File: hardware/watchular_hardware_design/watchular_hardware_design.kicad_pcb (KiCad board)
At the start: 4 copper layers, 55.5 x 22.9 mm, 90 parts, among them J1 USB4105-GF-A, J2 665102131822, J3 TSW-116-07-H-S, J4 TSW-116-07-H-S, Q1 BSS123, Q2 BSS123, Q3 BSS123, Q4 BSS123, T1 DMG1013UW-7, U1 MCP73832T-2DCI/OT, U2 ESP32-C3FH4, U3 MIC5524-3.3YMT-TZ, U4 W25Q16JVSSIQ, U5 TL3305AF260QG, U6 TL3305AF260QG, Y1 40MHz

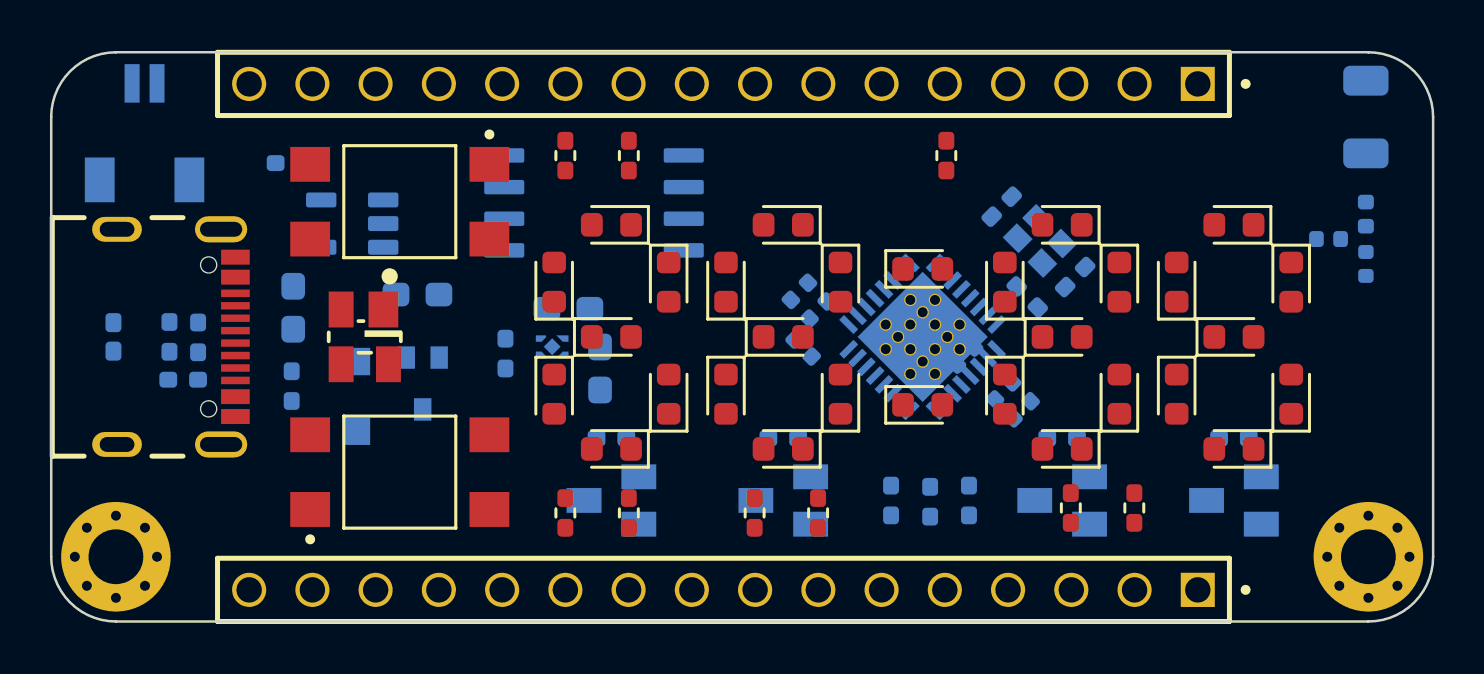
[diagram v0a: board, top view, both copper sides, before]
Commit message: Let the routing begin.
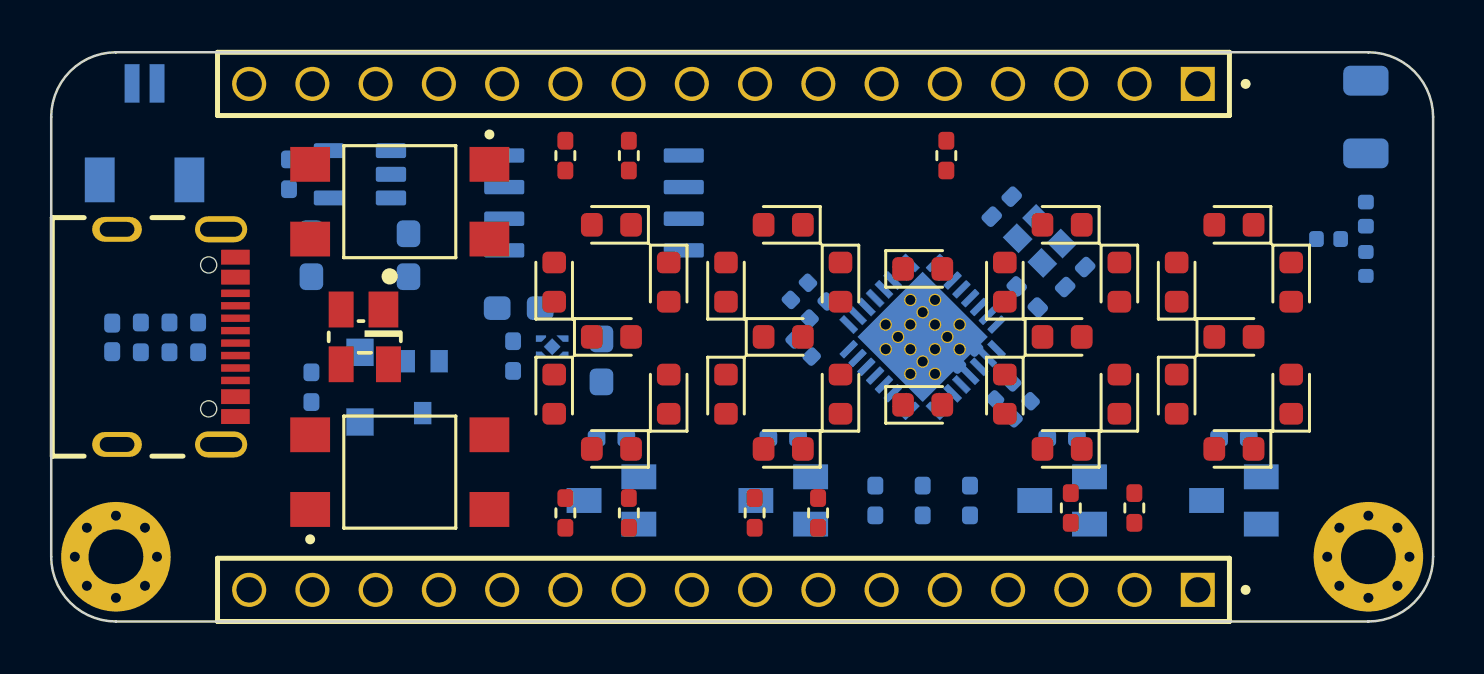
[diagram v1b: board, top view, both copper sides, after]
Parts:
- moved R5 2.40 mm to (93.6, 121.5), turned to 90 degrees
- moved C1 2.23 mm to (100.5, 118.2)
- moved U1 2.00 mm to (102.4, 114.9)
- moved C3 2.00 mm to (108.8, 120.3), turned to 180 degrees
- moved C2 1.62 mm to (104.3, 118.2), turned to -90 degrees
- moved R6 0.79 mm to (100.5, 123.5)
- moved R8 0.63 mm to (123.1, 128.0)
- moved R4 0.45 mm to (99.5, 114.9), turned to -90 degrees
- moved D1 0.40 mm to (102.4, 123.5)
- moved C6 0.33 mm to (112.1, 122.4)
- moved R7 0.32 mm to (108.5, 122.2)
- moved R3 0.30 mm to (125.0, 128.0)
- moved T1 0.15 mm to (104.9, 123.5)
- moved D2 0.05 mm to (92.5, 121.5)
